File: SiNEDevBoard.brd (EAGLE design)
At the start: 40 x 45 mm, 37 parts, among them IC1 ATTINY24/44/84-SSU, IC2 74HC164D, J1 AVR_SPI_PRG_6NS

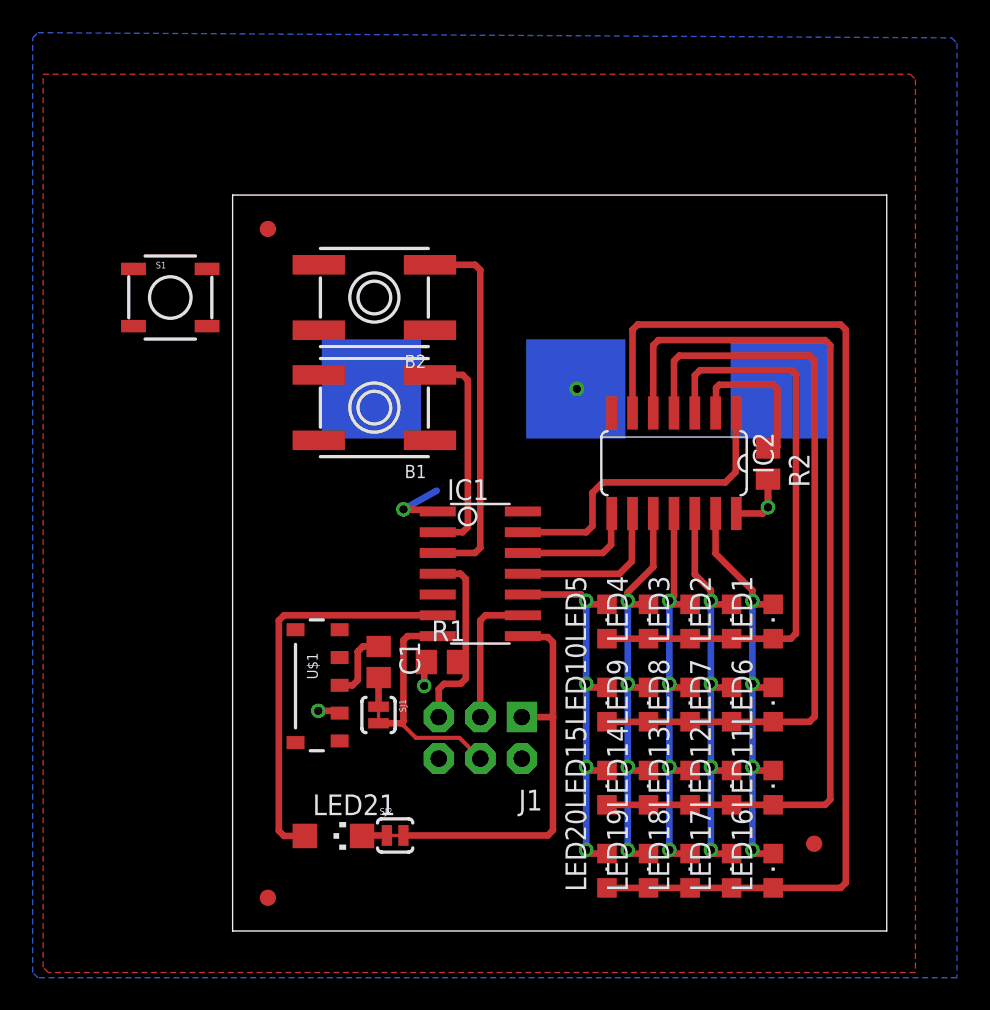
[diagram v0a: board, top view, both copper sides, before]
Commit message: DevBoard V0.3
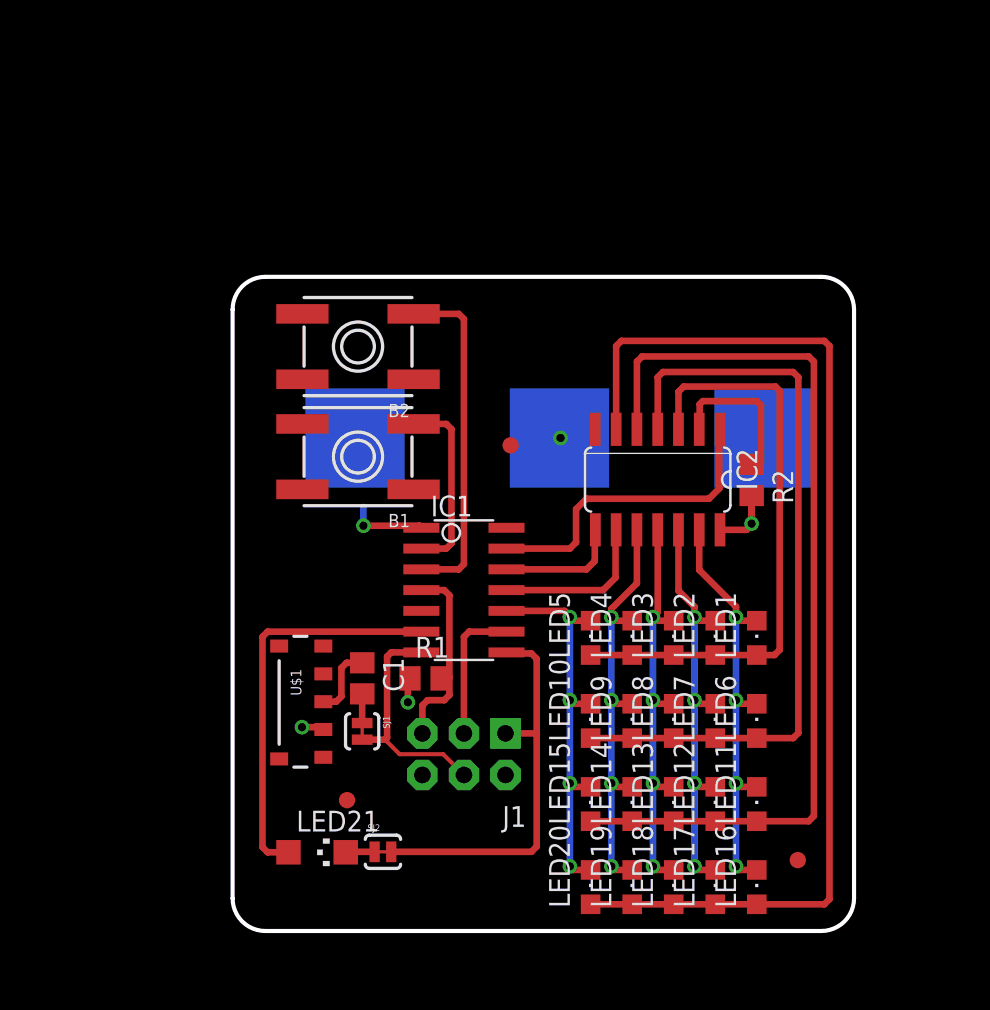
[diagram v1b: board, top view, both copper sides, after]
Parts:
- removed S1: (no value), CISECO eaglecad designs:TACTILE_SWITCH_SMD_LWK
- C1: value (none) -> 0603 100nF
- R1, R2: value (none) -> 0603 10K
- moved JP2 19.9 mm to (17.0, 29.7)
- moved JP1 7.68 mm to (7.00, 8.00)
- moved B2 3.16 mm to (7.67, 35.7)
- moved BAT1 3.16 mm to (20.0, 30.1)
- moved B1 3.16 mm to (7.67, 29.0)
- moved C1 1.41 mm to (7.93, 15.4)
- moved IC1 1.41 mm to (14.1, 20.8)
- moved IC2 1.41 mm to (26.0, 27.6)
- moved J1 1.41 mm to (14.1, 10.8)
- moved JP3 1.41 mm to (34.6, 4.33)
- moved LED1 1.41 mm to (32.1, 17.9)
- moved LED10 1.41 mm to (21.9, 12.8)
- moved LED11 1.41 mm to (32.1, 7.76)
- moved LED12 1.41 mm to (29.5, 7.76)
- moved LED13 1.41 mm to (27.0, 7.76)
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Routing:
- net BTN2: track 22.9 -> 20.9 mm
- net BTN1: track 13.4 -> 11.4 mm
- net GND: track 0.20 -> 2.07 mm
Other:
- board size 40 x 45 mm -> 38 x 40 mm
- board text added: "EMWave 2013"
- board text added: "SiNE DevBoard"
- board text added: "v0.3"

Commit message: DevBoard V0.4
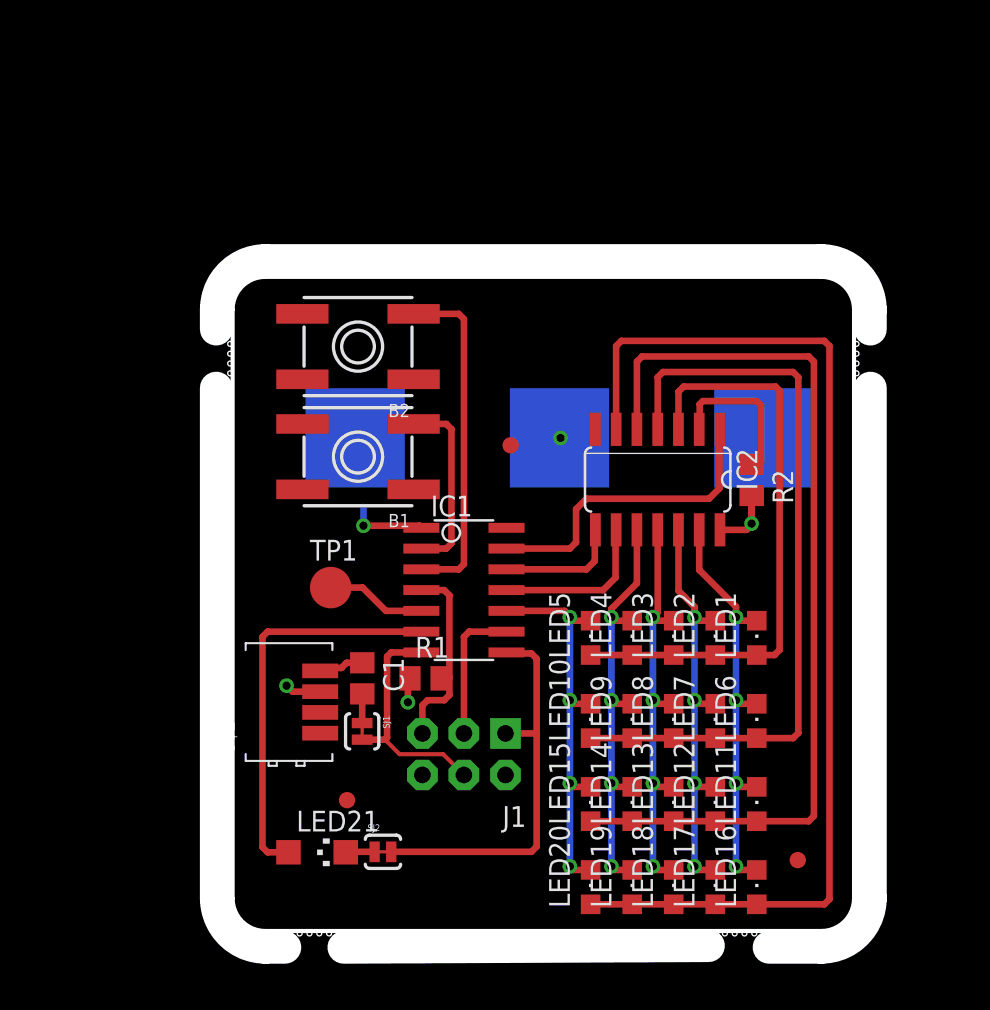
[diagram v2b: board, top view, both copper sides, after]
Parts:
- removed U$1: IRRECEIVERSMD, SparkFun:TSOP8523
- added TP1: TPB2,54, CISECO eaglecad designs:B2,54
- added U$2: IR-RECEIVER, CISECO eaglecad designs:TSOP35X
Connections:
- removed net N$2: IC1.5
- new net TESTPAD: IC1.5, TP1.TP
- net GND: now also U$2.1, U$2.2; no longer U$1.1, U$1.4, U$1.5
- net N$6: now also U$2.4; no longer U$1.3
- net VCC: now also U$2.3; no longer U$1.2
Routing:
- net TESTPAD: track 0.00 -> 6.13 mm
- net N$6: track 4.39 -> 3.36 mm
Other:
- board size 38 x 40 mm -> 40 x 42 mm
- board text added: "v0.4"
- board text removed: "v0.3"
